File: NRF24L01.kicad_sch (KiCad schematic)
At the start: 19 parts, among them U3 NRF24L01, Y2 16MHz

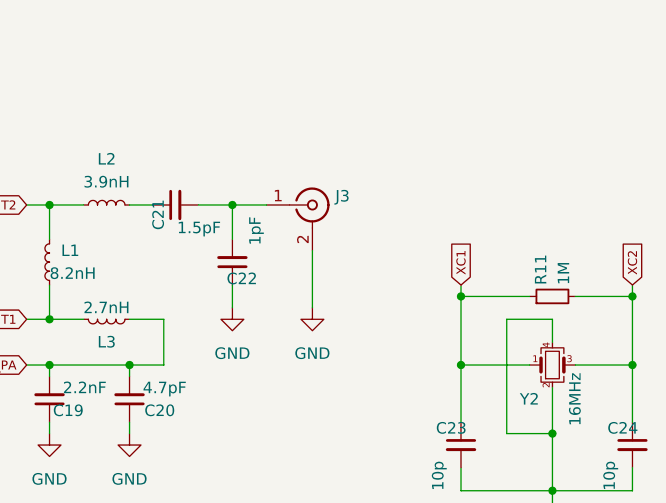
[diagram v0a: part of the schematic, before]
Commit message: updated pictures
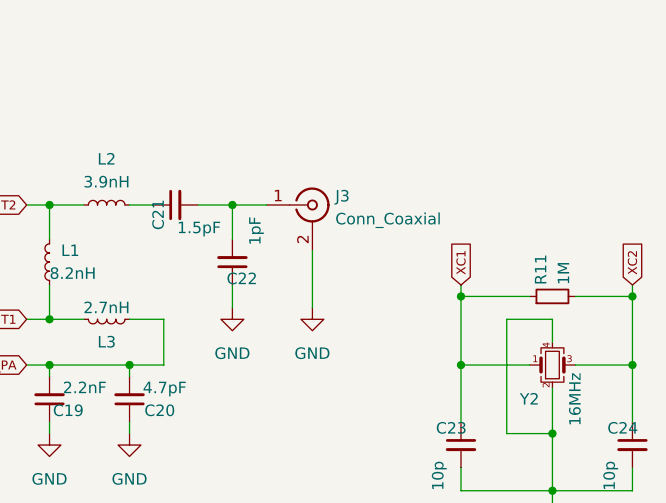
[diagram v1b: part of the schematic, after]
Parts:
- J3: value (none) -> Conn_Coaxial; footprint (none) -> Connector_Coaxial:SMA_Samtec_SMA-J-P-X-ST-EM1_EdgeMount
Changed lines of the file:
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@@
       (effects (font (size 1.27 1.27)) (justify left))
     )
-    (property "Value" "" (id 1) (at 196.85 77.7631 0)
+    (property "Value" "Conn_Coaxial" (id 1) (at 196.85 77.7631 0)
       (effects (font (size 1.27 1.27)) (justify left))
     )
-    (property "Footprint" "" (id 2) (at 194.31 76.2 0)
+    (property "Footprint" "Connector_Coaxial:SMA_Samtec_SMA-J-P-X-ST-EM1_EdgeMount" (id 2) (at 194.31 76.2 0)
       (effects (font (size 1.27 1.27)) hide)
     )
